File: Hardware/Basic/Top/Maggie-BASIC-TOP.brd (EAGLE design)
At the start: 37.9 x 38.1 mm, 59 parts, among them SW1 SWITCH.MOM, SW2 SWITCH.MOM, U2 NRF52832_MODULE_MDBT42, U4 FT231XS

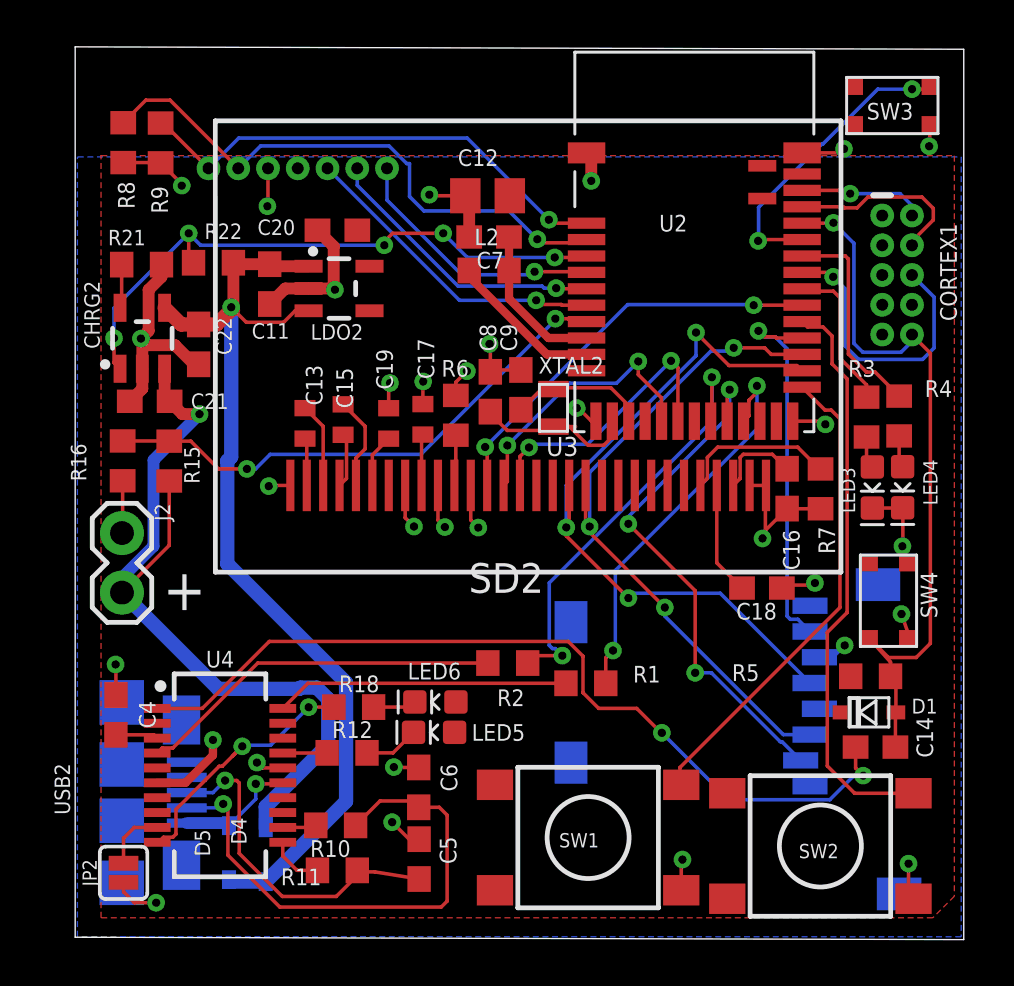
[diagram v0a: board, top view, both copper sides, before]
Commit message: check
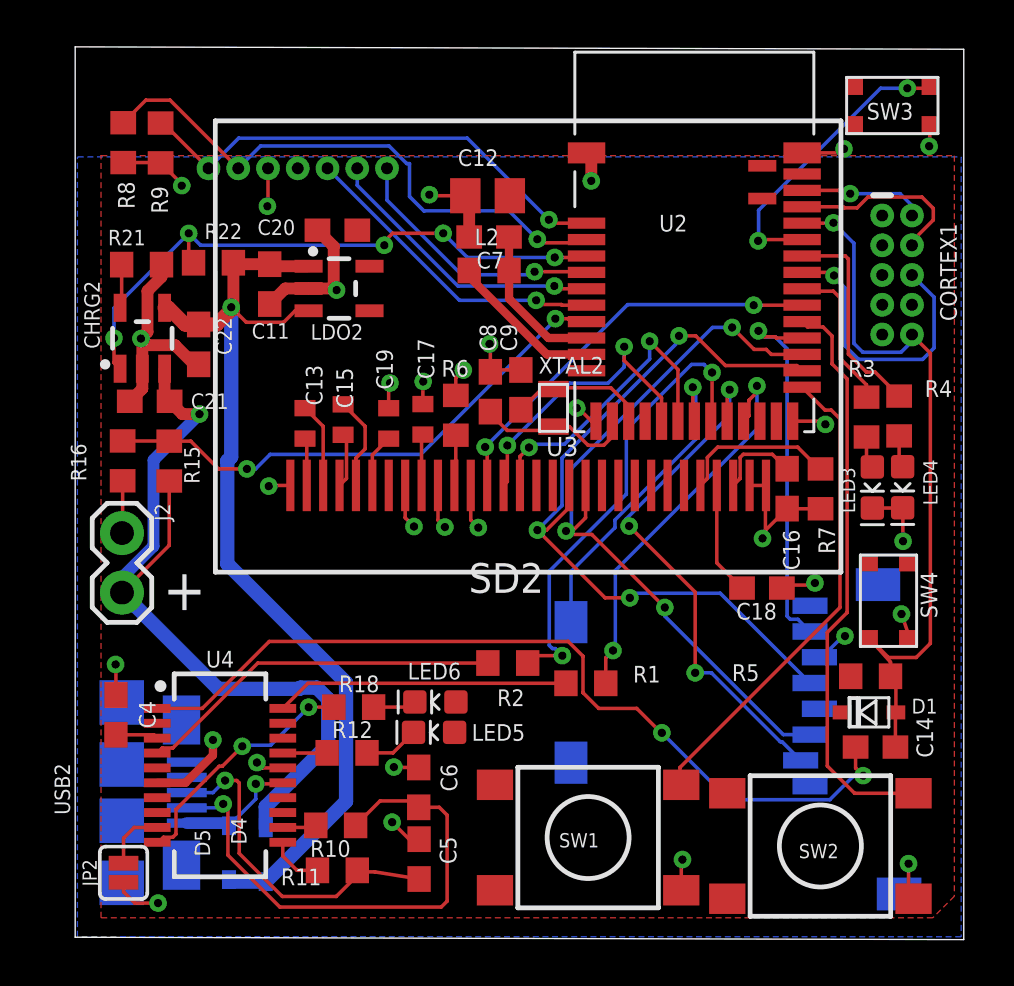
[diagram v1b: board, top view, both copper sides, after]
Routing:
- net D5/CD1: track 0.00 -> 13.8 mm, vias 0 -> 1
- net MOSI: track 29.0 -> 32.3 mm
- net SCK: track 31.2 -> 33.9 mm
- net TXD.NRF: track 18.6 -> 20.0 mm
- net D4/DCOLED: track 12.2 -> 13.2 mm
- net D3/RESETOLED: track 11.8 -> 12.9 mm
- net N$4: track 7.84 -> 6.90 mm
- net TXLED: track 11.2 -> 10.6 mm
